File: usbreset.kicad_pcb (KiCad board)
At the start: 2 copper layers, 39.1 x 22.9 mm, 13 parts, among them J1 USB_C_PowerSource, J2 USB_C_PowerSink, J3 USB3_A_Plug, J4 USB3_A_Receptacle, Q1 SI2393DS, SW1 EN_USBA, SW2 SW_Push, SW3 SW_Push

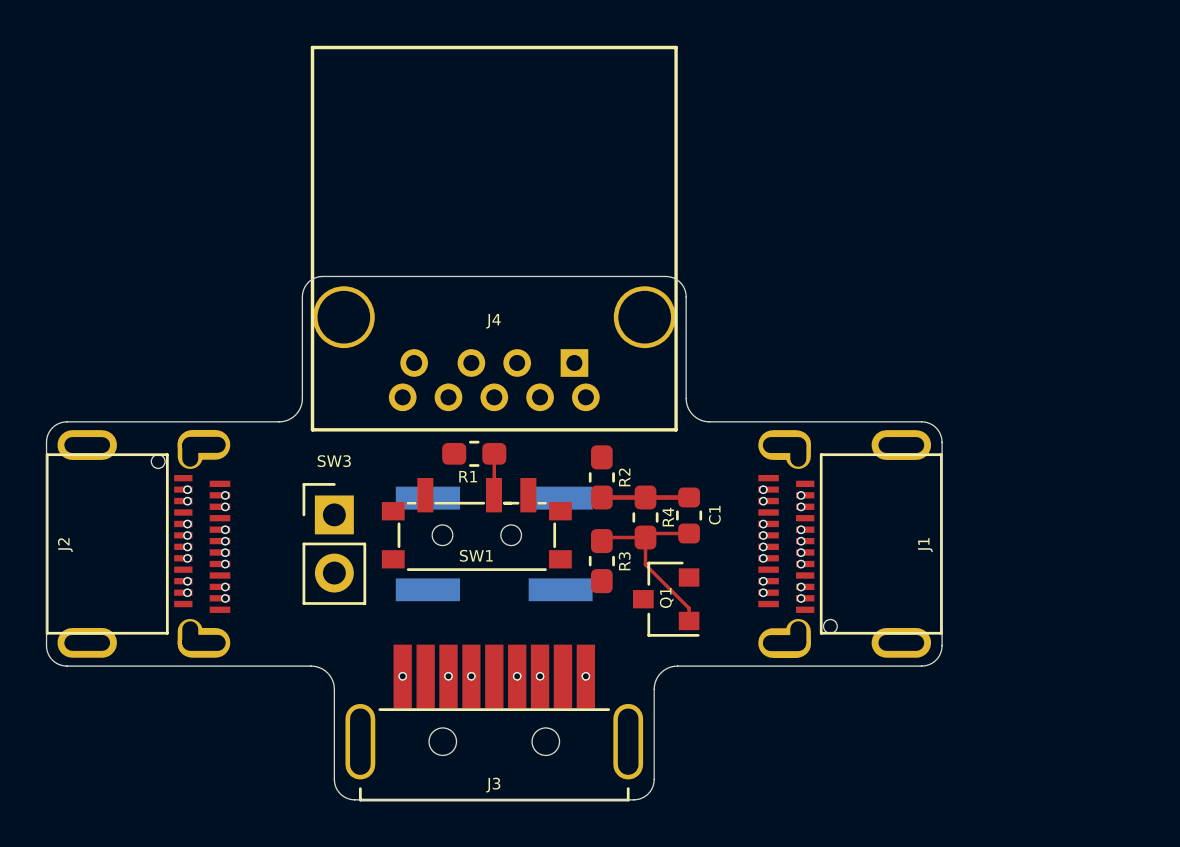
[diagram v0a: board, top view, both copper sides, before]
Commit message: Route most connections
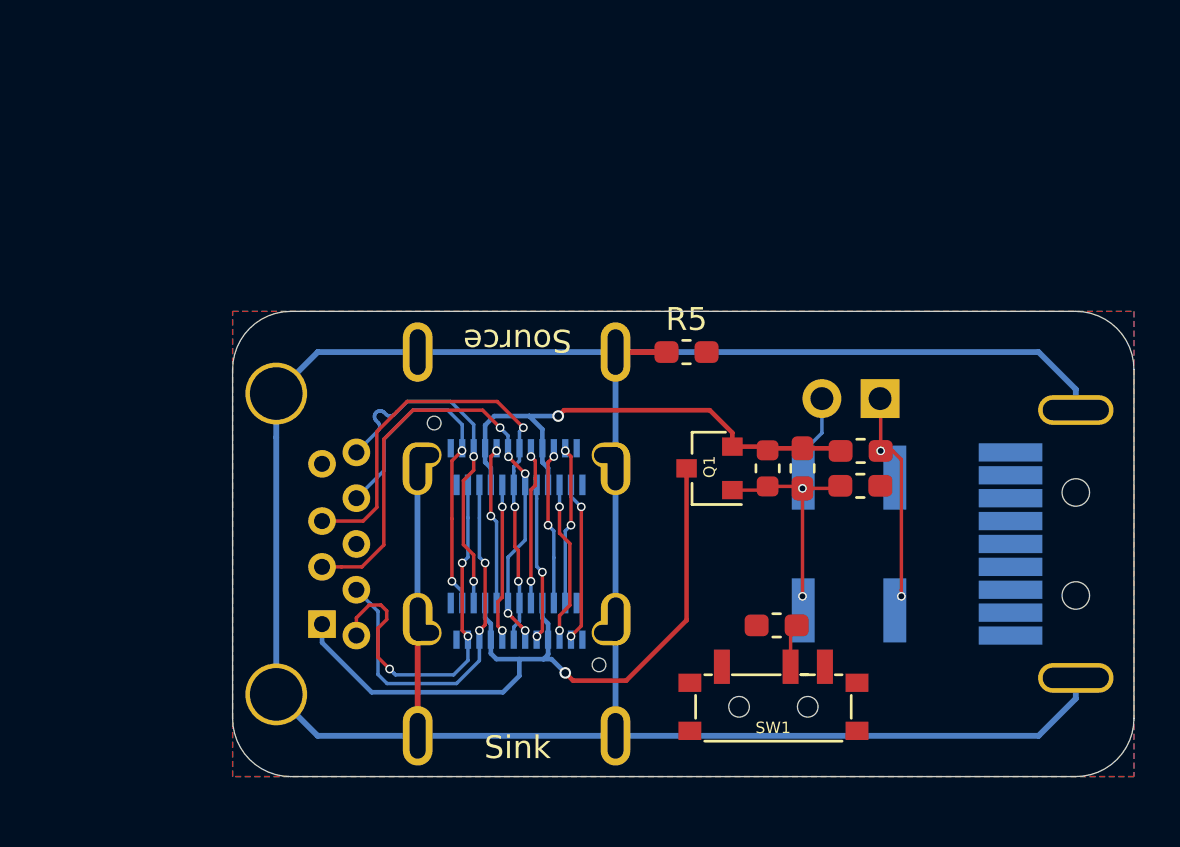
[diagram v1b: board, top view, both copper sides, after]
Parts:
- added R5: 0, Resistor_SMD:R_0603_1608Metric_Pad1.05x0.95mm_HandSolder, F.Cu at (160.8, 94.5)
- J1, J2, J3, J4, SW3: moved to B.Cu
- moved J3 26.8 mm to (177.8, 102.9), turned to 270 degrees
- moved SW3 24.4 mm to (169.2, 96.5), turned to 90 degrees
- moved J2 20.5 mm to (153.4, 111.2), turned to 180 degrees
- moved J1 18.8 mm to (153.4, 94.5), turned to 0 degrees
- moved J4 18.6 mm to (139.4, 102.9), turned to 90 degrees
- moved SW2 15.5 mm to (167.9, 102.9), turned to 90 degrees
- moved R1 15.2 mm to (164.7, 106.4)
- moved SW1 15.0 mm to (164.6, 110.0)
- moved R3 11.8 mm to (168.4, 100.3), turned to 0 degrees
- moved R2 11.4 mm to (168.4, 98.8), turned to 0 degrees
- moved R4 7.19 mm to (165.9, 99.6)
- moved Q1 6.02 mm to (161.8, 99.6)
- moved C1 4.00 mm to (164.3, 99.6)
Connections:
- J1 pad A10: Net-(J1-PadA10) -> /RX2-
- J1 pad A11: Net-(J1-PadA11) -> /RX2+
- J1 pad A2: Net-(J1-PadA2) -> /TX1+
- J1 pad A3: Net-(J1-PadA3) -> /TX1-
- J1 pad A5: Net-(J1-PadA5) -> /CC1
- J1 pad A6: Net-(J1-PadA6) -> /D+
- J1 pad A7: Net-(J1-PadA7) -> /D-
- J1 pad A8: Net-(J1-PadA8) -> /SBU1
- J1 pad B10: Net-(J1-PadB10) -> /RX1-
- J1 pad B11: Net-(J1-PadB11) -> /RX1+
- J1 pad B2: Net-(J1-PadB2) -> /TX2+
- J1 pad B3: Net-(J1-PadB3) -> /TX2-
- J1 pad B5: Net-(J1-PadB5) -> /CC2
- J1 pad B6: Net-(J1-PadB6) -> /D+
- J1 pad B7: Net-(J1-PadB7) -> /D-
- J1 pad B8: Net-(J1-PadB8) -> /SBU2
- J2 pad A10: Net-(J2-PadA10) -> /RX1-
- J2 pad A11: Net-(J1-PadA11) -> /RX1+
- J2 pad A2: Net-(J1-PadA2) -> /TX2+
- J2 pad A3: Net-(J1-PadA3) -> /TX2-
- J2 pad A5: Net-(J1-PadA5) -> /CC2
- J2 pad A6: Net-(J1-PadA6) -> /D+
- J2 pad A7: Net-(J1-PadA7) -> /D-
- J2 pad A8: Net-(J1-PadA8) -> /SBU2
- J2 pad B10: Net-(J1-PadB10) -> /RX2-
- J2 pad B11: Net-(J1-PadB11) -> /RX2+
- J2 pad B2: Net-(J1-PadB2) -> /TX1+
- J2 pad B3: Net-(J1-PadB3) -> /TX1-
- J2 pad B5: Net-(J1-PadB5) -> /CC1
- J2 pad B6: Net-(J1-PadB6) -> /D+
- J2 pad B7: Net-(J1-PadB7) -> /D-
- J2 pad B8: Net-(J1-PadB8) -> /SBU1
- J3 pad 2: Net-(J1-PadA7) -> /D-
- J3 pad 3: Net-(J1-PadA6) -> /D+
- J3 pad 5: Net-(J1-PadB10) -> /RX1-
- J3 pad 6: Net-(J1-PadB11) -> /RX1+
- J3 pad 8: Net-(J1-PadA3) -> /TX1-
- J3 pad 9: Net-(J1-PadA2) -> /TX1+
- J4 pad 2: Net-(J1-PadA7) -> /D-
- J4 pad 3: Net-(J1-PadA6) -> /D+
- J4 pad 5: Net-(J1-PadB10) -> /RX1-
- J4 pad 6: Net-(J1-PadB11) -> /RX1+
- J4 pad 8: Net-(J1-PadA3) -> /TX1-
- J4 pad 9: Net-(J1-PadA2) -> /TX1+
- SW1 pad 1: Net-(J1-PadA5) -> /CC1
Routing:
- net SHIELD: track 0.00 -> 118.8 mm
- net /VBUS_SINK: track 0.00 -> 33.1 mm, vias 0 -> 1
- net /D-: track 0.00 -> 23.1 mm, vias 0 -> 5
- net /D+: track 0.00 -> 23.0 mm, vias 0 -> 3
- net VBUS: track 3.81 -> 23.0 mm, vias 0 -> 1
- net /TX1+: track 0.00 -> 16.9 mm, vias 0 -> 3
- net /TX1-: track 0.00 -> 16.6 mm, vias 0 -> 2
- net /RX1+: track 0.00 -> 15.3 mm, vias 0 -> 2
- net /RX1-: track 0.00 -> 15.1 mm, vias 0 -> 2
- net Net-(R2-Pad2): track 0.00 -> 11.6 mm, vias 0 -> 2
- net /RX2+: track 0.00 -> 6.98 mm, vias 0 -> 2
- net /TX2+: track 0.00 -> 6.86 mm, vias 0 -> 2
- net /SBU2: track 0.00 -> 6.86 mm, vias 0 -> 2
- net /SBU1: track 0.00 -> 6.82 mm, vias 0 -> 2
- net /RX2-: track 0.00 -> 6.73 mm, vias 0 -> 2
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- added copper zone on B.Cu, net GND
- added copper zone on F.Cu, net GND
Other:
- board size 39.1 x 22.9 mm -> 39.4 x 20.3 mm
- net class Default: clearance 0.16 -> 0.1524
- net class Shield added: clearance 0.16, trace_width 0.254, via_dia 0.508, via_drill 0.3302
- rule trace_clearance: 0.16 -> 0.1524
- board text added: "Sink"
- board text added: "Source"
